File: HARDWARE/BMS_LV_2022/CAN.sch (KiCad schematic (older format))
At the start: 10 parts, among them U3 ATA6561-GAQW-N

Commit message: Electrical Rules Checker fixes
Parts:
- removed FB2, FB4: 60R@100MHz, Inductor_SMD:L_0603_1608Metric, symbol Device:Ferrite_Bead_Small
- added FB2, FB3: 60R@100MHz, symbol FerriteBead:Ferrite_Bead_Small
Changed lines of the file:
@@
 CAN-TX
-$Comp
-L Device:Ferrite_Bead_Small FB?
-U 1 1 61A2B363
-P 4300 3850
-AR Path="/61A064B3/61A2B363" Ref="FB?"  Part="1"
-AR Path="/61A14ADD/61A2B363" Ref="FB4"  Part="1"
-AR Path="/61A9D384/61A2B363" Ref="FB6"  Part="1"
-AR Path="/61F4D531/61A2B363" Ref="FB6"  Part="1"
-F 0 "FB6" H 4400 3896 50  0000 L CNN
-F 1 "60R@100MHz" H 4400 3805 50  0000 L CNN
-F 2 "Inductor_SMD:L_0603_1608Metric" V 4230 3850 50  0001 C CNN
-F 3 "~" H 4300 3850 50  0001 C CNN
-F 4 "" H 4300 3850 50  0001 C CNN "LCSC"
-	1    4300 3850
-	-1   0    0    -1
-$EndComp
 $Comp
 L power:+3V3 #PWR?
@@
 Wire Wire Line
 	2350 4400 2350 4350
-$Comp
-L Device:Ferrite_Bead_Small FB?
-U 1 1 61AA449D
-P 2350 3850
-AR Path="/61A064B3/61AA449D" Ref="FB?"  Part="1"
-AR Path="/61A14ADD/61AA449D" Ref="FB2"  Part="1"
-AR Path="/61A9D384/61AA449D" Ref="FB5"  Part="1"
-AR Path="/61F4D531/61AA449D" Ref="FB5"  Part="1"
-F 0 "FB5" H 2450 3896 50  0000 L CNN
-F 1 "60R@100MHz" H 2450 3805 50  0000 L CNN
-F 2 "Inductor_SMD:L_0603_1608Metric" V 2280 3850 50  0001 C CNN
-F 3 "~" H 2350 3850 50  0001 C CNN
-F 4 "" H 2350 3850 50  0001 C CNN "LCSC"
-	1    2350 3850
-	1    0    0    -1
-$EndComp
 Wire Wire Line
 	2350 3650 2350 3750
@@
 EndData
 $EndBitmap
+$Comp
+L FerriteBead:Ferrite_Bead_Small FB2
+U 1 1 61BF4101
+P 4300 3850
+F 0 "FB2" H 4400 3800 50  0000 L CNN
+F 1 "60R@100MHz" H 4400 3900 50  0000 L CNN
+F 2 "" V 4230 3850 50  0001 C CNN
+F 3 "~" H 4300 3850 50  0001 C CNN
+	1    4300 3850
+	-1   0    0    1
+$EndComp
+$Comp
+L FerriteBead:Ferrite_Bead_Small FB3
+U 1 1 61C02070
+P 2350 3850
+F 0 "FB3" H 2244 3804 50  0000 R CNN
+F 1 "60R@100MHz" H 2244 3895 50  0000 R CNN
+F 2 "" V 2280 3850 50  0001 C CNN
+F 3 "~" H 2350 3850 50  0001 C CNN
+	1    2350 3850
+	1    0    0    1
+$EndComp
 $EndSCHEMATC

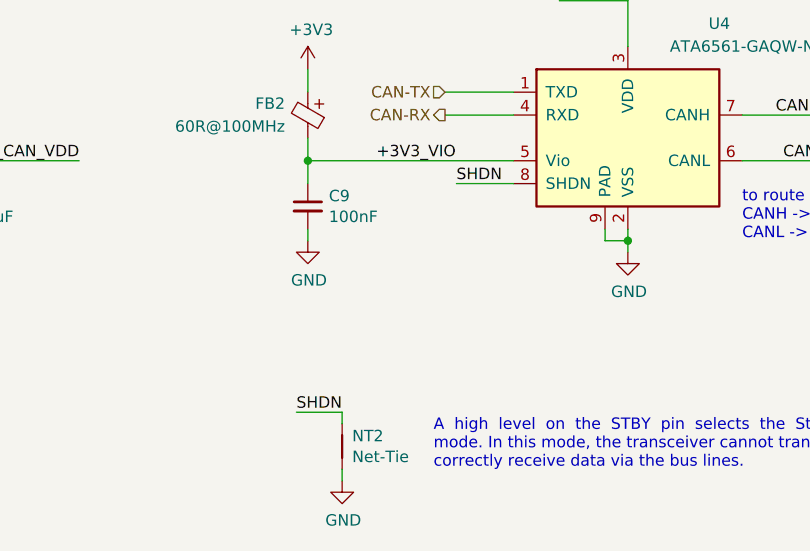
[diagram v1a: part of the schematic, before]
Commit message: Most of the footprints added
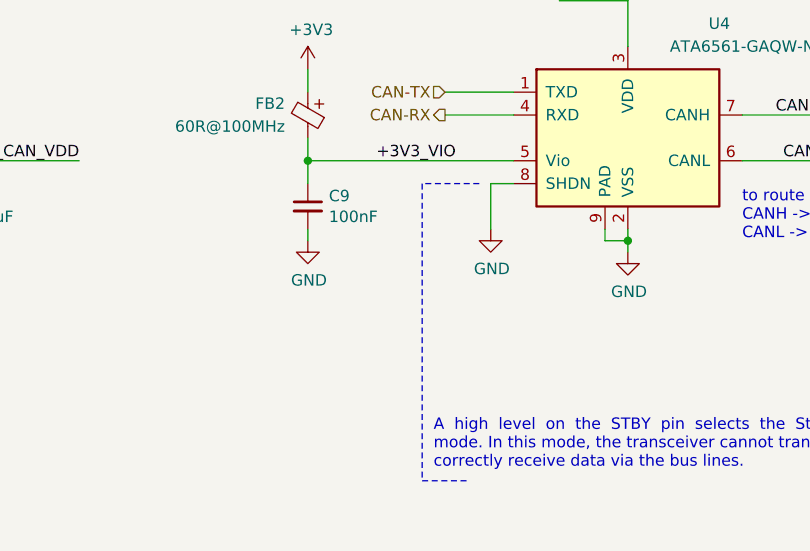
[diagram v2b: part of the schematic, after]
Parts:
- removed NT1: Net-Tie, symbol Device:Net-Tie_2
- C4, C5, C6: footprint (none) -> Capacitor_SMD:C_0603_1608Metric
- FB2, FB3: footprint (none) -> Inductor_SMD:L_0603_1608Metric
- R3: footprint (none) -> Resistor_SMD:R_0603_1608Metric
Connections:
- net SHDN is gone; now on net GND: U3.8 (SHDN)
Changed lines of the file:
@@
 F 0 "C9" H 4392 4296 50  0000 L CNN
 F 1 "100nF" H 4392 4205 50  0000 L CNN
-F 2 "" H 4300 4250 50  0001 C CNN
+F 2 "Capacitor_SMD:C_0603_1608Metric" H 4300 4250 50  0001 C CNN
 F 3 "~" H 4300 4250 50  0001 C CNN
 	1    4300 4250
@@
 F 0 "R4" H 8970 4146 50  0000 L CNN
 F 1 "120R" H 8970 4055 50  0000 L CNN
-F 2 "" V 8830 4100 50  0001 C CNN
+F 2 "Resistor_SMD:R_0603_1608Metric" V 8830 4100 50  0001 C CNN
 F 3 "~" H 8900 4100 50  0001 C CNN
 	1    8900 4100
@@
 Text Notes 4850 5400 0    50   ~ 0
 A  high  level  on  the  STBY  pin  selects  the  Standby\nmode. In this mode, the transceiver cannot transmit or\ncorrectly receive data via the bus lines.
-Wire Wire Line
-	4950 4150 5200 4150
-Text Label 4950 4150 0    50   ~ 0
-SHDN
-Text Label 4250 5150 0    50   ~ 0
-SHDN
-Wire Wire Line
-	4250 5150 4450 5150
-Wire Wire Line
-	4450 5150 4450 5200
-Wire Wire Line
-	4450 5400 4450 5450
 $Comp
 L power:GND #PWR014
 U 1 1 61A94FC7
-P 4450 5450
+P 5100 4350
 AR Path="/61A14ADD/61A94FC7" Ref="#PWR014"  Part="1"
 AR Path="/61A9D384/61A94FC7" Ref="#PWR021"  Part="1"
 AR Path="/61F4D531/61A94FC7" Ref="#PWR021"  Part="1"
-F 0 "#PWR021" H 4450 5200 50  0001 C CNN
-F 1 "GND" H 4455 5277 50  0000 C CNN
-F 2 "" H 4450 5450 50  0001 C CNN
-F 3 "" H 4450 5450 50  0001 C CNN
-	1    4450 5450
+F 0 "#PWR021" H 5100 4100 50  0001 C CNN
+F 1 "GND" H 5105 4177 50  0000 C CNN
+F 2 "" H 5100 4350 50  0001 C CNN
+F 3 "" H 5100 4350 50  0001 C CNN
+	1    5100 4350
 	1    0    0    -1
-$EndComp
-$Comp
-L Device:Net-Tie_2 NT1
-U 1 1 61A96008
-P 4450 5300
-AR Path="/61A14ADD/61A96008" Ref="NT1"  Part="1"
-AR Path="/61A9D384/61A96008" Ref="NT2"  Part="1"
-AR Path="/61F4D531/61A96008" Ref="NT2"  Part="1"
-F 0 "NT2" V 4404 5344 50  0000 L CNN
-F 1 "Net-Tie" V 4495 5344 50  0000 L CNN
-F 2 "" H 4450 5300 50  0001 C CNN
-F 3 "~" H 4450 5300 50  0001 C CNN
-	1    4450 5300
-	0    1    1    0
 $EndComp
 Text Label 3300 4050 2    50   ~ 0
@@
 F 0 "C7" H 2442 4296 50  0000 L CNN
 F 1 "100nF" H 2442 4205 50  0000 L CNN
-F 2 "" H 2350 4250 50  0001 C CNN
+F 2 "Capacitor_SMD:C_0603_1608Metric" H 2350 4250 50  0001 C CNN
 F 3 "~" H 2350 4250 50  0001 C CNN
 	1    2350 4250
@@
 F 0 "C8" H 2842 4296 50  0000 L CNN
 F 1 "10uF" H 2842 4205 50  0000 L CNN
-F 2 "" H 2750 4250 50  0001 C CNN
+F 2 "Capacitor_SMD:C_0603_1608Metric" H 2750 4250 50  0001 C CNN
 F 3 "~" H 2750 4250 50  0001 C CNN
 	1    2750 4250
@@
 F 0 "FB2" H 4400 3800 50  0000 L CNN
 F 1 "60R@100MHz" H 4400 3900 50  0000 L CNN
-F 2 "" V 4230 3850 50  0001 C CNN
+F 2 "Inductor_SMD:L_0603_1608Metric" V 4230 3850 50  0001 C CNN
 F 3 "~" H 4300 3850 50  0001 C CNN
 	1    4300 3850
@@
 F 0 "FB3" H 2244 3804 50  0000 R CNN
 F 1 "60R@100MHz" H 2244 3895 50  0000 R CNN
-F 2 "" V 2280 3850 50  0001 C CNN
+F 2 "Inductor_SMD:L_0603_1608Metric" V 2280 3850 50  0001 C CNN
 F 3 "~" H 2350 3850 50  0001 C CNN
 	1    2350 3850
 	1    0    0    1
 $EndComp
+Wire Wire Line
+	5100 4150 5100 4350
+Wire Wire Line
+	5100 4150 5200 4150
+Wire Notes Line
+	5050 4150 4800 4150
+Wire Notes Line
+	4800 5450 5000 5450
+Wire Notes Line
+	4800 4150 4800 5450
 $EndSCHEMATC

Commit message: Some footprint changes
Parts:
- FB2, FB3: symbol FerriteBead:Ferrite_Bead_Small -> BMS_LV_2022-rescue:Ferrite_Bead_Small-FerriteBead
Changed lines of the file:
@@
 $EndBitmap
 $Comp
-L FerriteBead:Ferrite_Bead_Small FB2
+L BMS_LV_2022-rescue:Ferrite_Bead_Small-FerriteBead FB2
 U 1 1 61BF4101
 P 4300 3850
+AR Path="/61BF4101" Ref="FB2"  Part="1"
+AR Path="/61F4D531/61BF4101" Ref="FB2"  Part="1"
 F 0 "FB2" H 4400 3800 50  0000 L CNN
 F 1 "60R@100MHz" H 4400 3900 50  0000 L CNN
@@
 $EndComp
 $Comp
-L FerriteBead:Ferrite_Bead_Small FB3
+L BMS_LV_2022-rescue:Ferrite_Bead_Small-FerriteBead FB3
 U 1 1 61C02070
 P 2350 3850
+AR Path="/61C02070" Ref="FB3"  Part="1"
+AR Path="/61F4D531/61C02070" Ref="FB3"  Part="1"
 F 0 "FB3" H 2244 3804 50  0000 R CNN
 F 1 "60R@100MHz" H 2244 3895 50  0000 R CNN
